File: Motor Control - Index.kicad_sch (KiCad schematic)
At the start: 8 parts, among them U10 TB9051FTG,EL

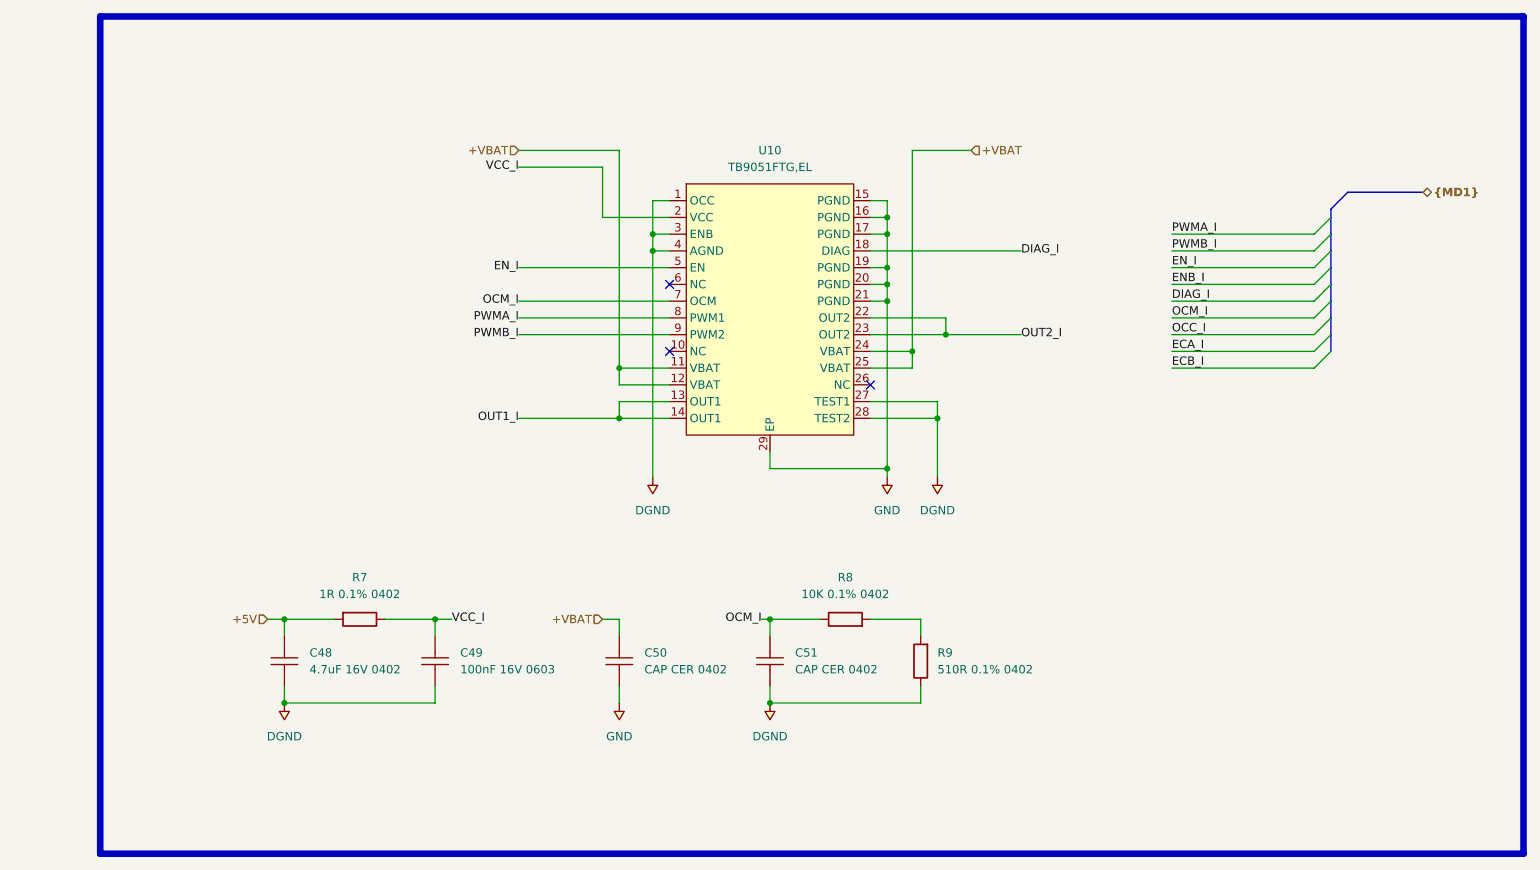
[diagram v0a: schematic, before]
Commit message: Update Schematic
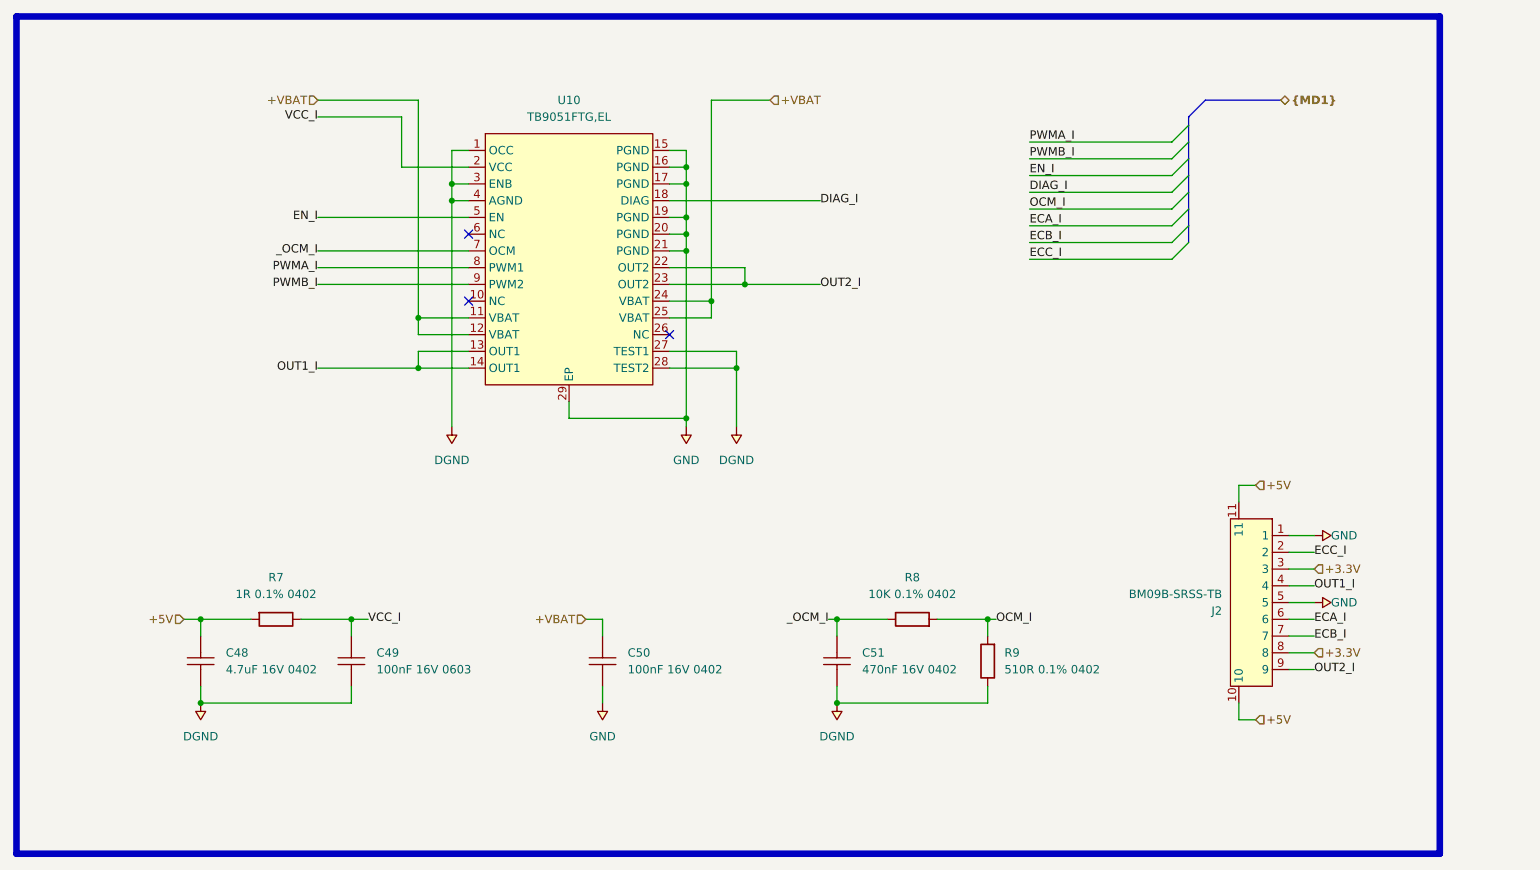
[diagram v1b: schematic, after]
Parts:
- added J2: BM09B-SRSS-TB, Duc:CONN-SMD_9P-P1.00_BM09B-SRSS-TB, symbol Duc-Connectors:BM09B-SRSS-TB
- C50: value CAP CER 0402 -> 100nF 16V 0402
- C51: value CAP CER 0402 -> 470nF 16V 0402
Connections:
- net +5V: now also J2.10, J2.11
- net ECA_I: now also J2.6
- net ECB_I: now also J2.7
- net GND: now also J2.1, J2.5
- net OCM_I: now also R8.1, R9.1; no longer C51.2, R8.2, U10.7 (OCM)
- net OUT1_I: now also J2.4
- net OUT2_I: now also J2.9
- new net +3.3V: J2.3, J2.8
- new net ECC_I: J2.2
- new net _OCM_I: C51.2, R8.2, U10.7 (OCM)
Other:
- moved on the sheet: C48, C49, C50, C51, R7, R8, R9, U10
